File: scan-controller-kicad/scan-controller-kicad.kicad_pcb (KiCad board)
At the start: 2 copper layers, 131.3 x 101.6 mm, 136 parts, among them CN1 24V in, CN2 Shaft Eye, CN3 Film End Eye, CN4 Fan, CN5 Motor, CN6 Lamp, J1 Raspi GPIO, J2 Raspi UART, J3 ICSP, J4 FTDI, J5 Shaft Eye, J6 Film End Eye, Q1 IRLML2502, Q2 IRLML6402, Q3 DMMT5401, Q4 DMG2305UX, Q5 SS8050, Q6 SS8050, Q7 IRF7470, SW1 Reset, SW10 Power, SW2 Lamp, SW3 Zoom, SW4 <<, SW5 <, SW6 Stop, SW7 >, SW8 >>, SW9 Rec, U1 ATmega328P, U2 74LVC14, U3 QRE1113, U4 QRE1113, U5 DRV8871DDA, U6 78L05, U7 XL4015, U8 TL431, U9 LM358, Y1 8MHz

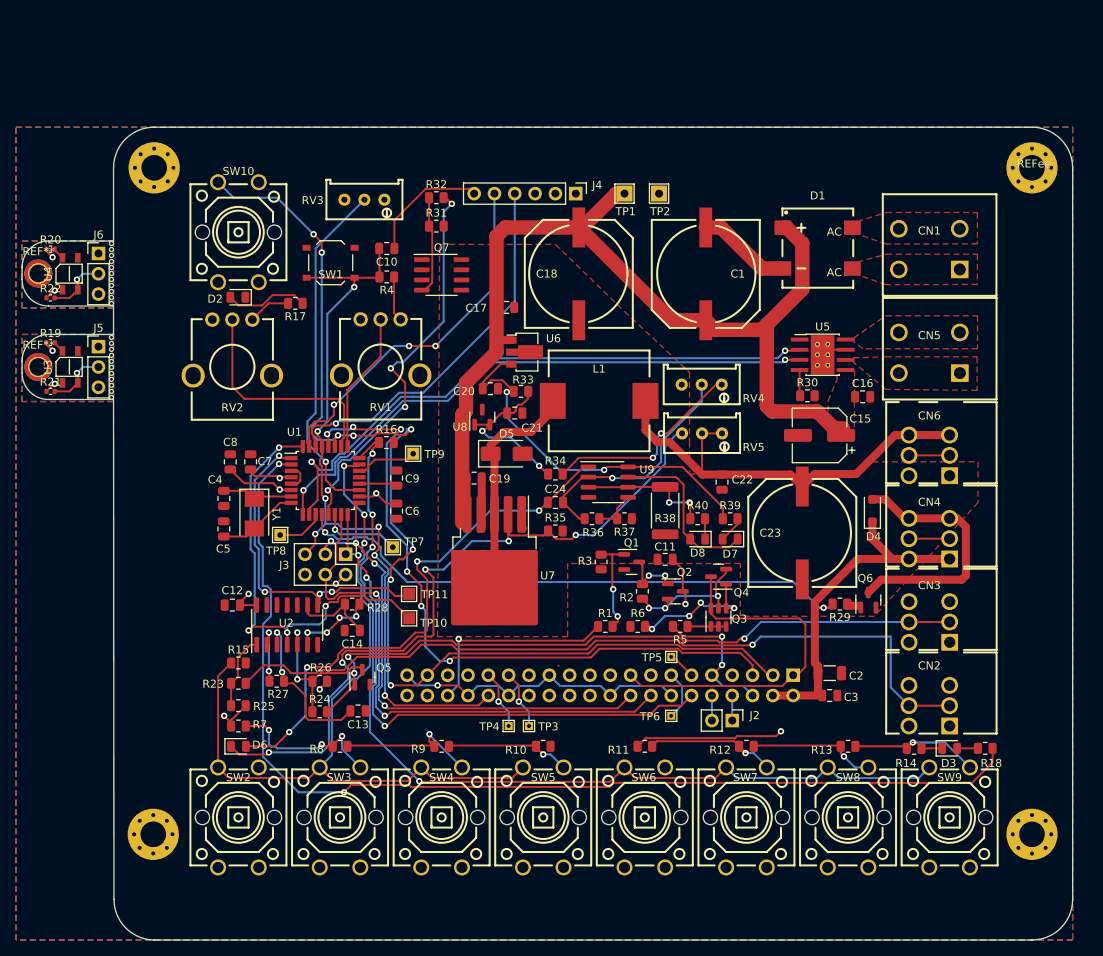
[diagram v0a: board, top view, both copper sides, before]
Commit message: Changes shape to hold the cehapo 5.0" Display as cover
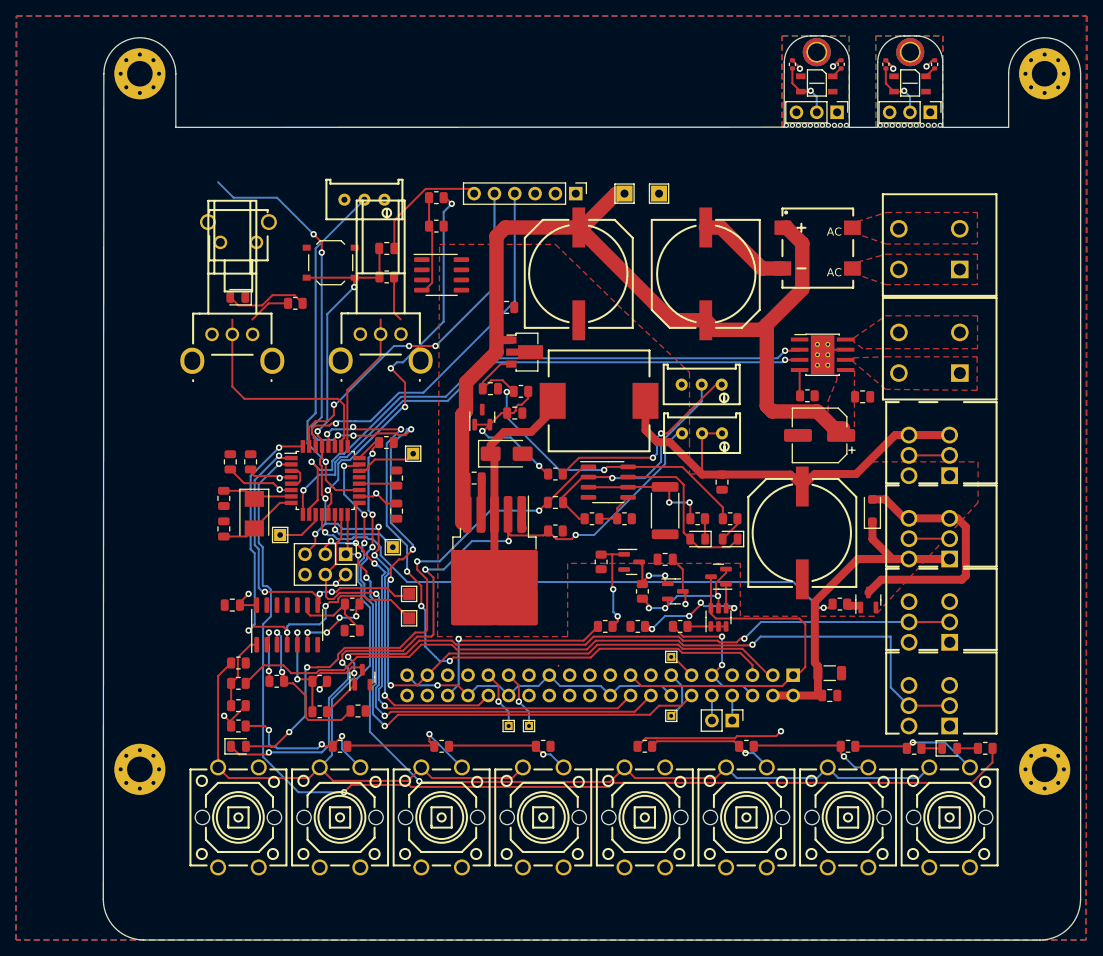
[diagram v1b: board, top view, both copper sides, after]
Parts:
- RV1, RV2: footprint easyeda2kicad:RES-ADJ-TH_RK09K1130AJ3 -> easyeda2kicad:RES-TH_RK09K1110A0J
- SW10: footprint easyeda2kicad:KEY-TH_4P-L12.0-W12.0-P5.0-LS12.5-EH-small -> easyeda2kicad:KEY-TH_4P-L7.3-W10.2-P4.50-LS7.0
- moved R20 112.9 mm to (224.1, 48.0), turned to -90 degrees
- moved REF** 112.4 mm to (221.0, 46.5), turned to -90 degrees
- moved R22 108.4 mm to (218.0, 48.0), turned to -90 degrees
- moved U4 107.9 mm to (221.0, 50.2), turned to 180 degrees
- moved J6 105.5 mm to (223.5, 54.0), turned to -90 degrees
- moved REF** 105.0 mm to (209.3, 46.5), turned to -90 degrees
- moved R19 104.8 mm to (212.4, 48.0), turned to -90 degrees
- moved REF** 101.5 mm to (221.0, 55.6), turned to 0 degrees
- moved R21 101.3 mm to (206.3, 48.0), turned to -90 degrees
- moved U3 100.2 mm to (209.3, 50.2), turned to 180 degrees
- moved J5 96.9 mm to (211.9, 54.0), turned to -90 degrees
- moved REF** 93.2 mm to (209.3, 55.6), turned to 0 degrees
- moved REF** 11.9 mm to (124.7, 49.2)
- moved REFee 11.9 mm to (237.8, 49.2)
- moved REF** 8.29 mm to (124.7, 136.2)
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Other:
- board size 131.3 x 101.6 mm -> 122.2 x 113 mm
